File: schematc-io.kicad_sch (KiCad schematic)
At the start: 50 parts, among them IC1 AD8544ARUZ-REEL, J4 Conn_01x04, U3 SN65HVD232

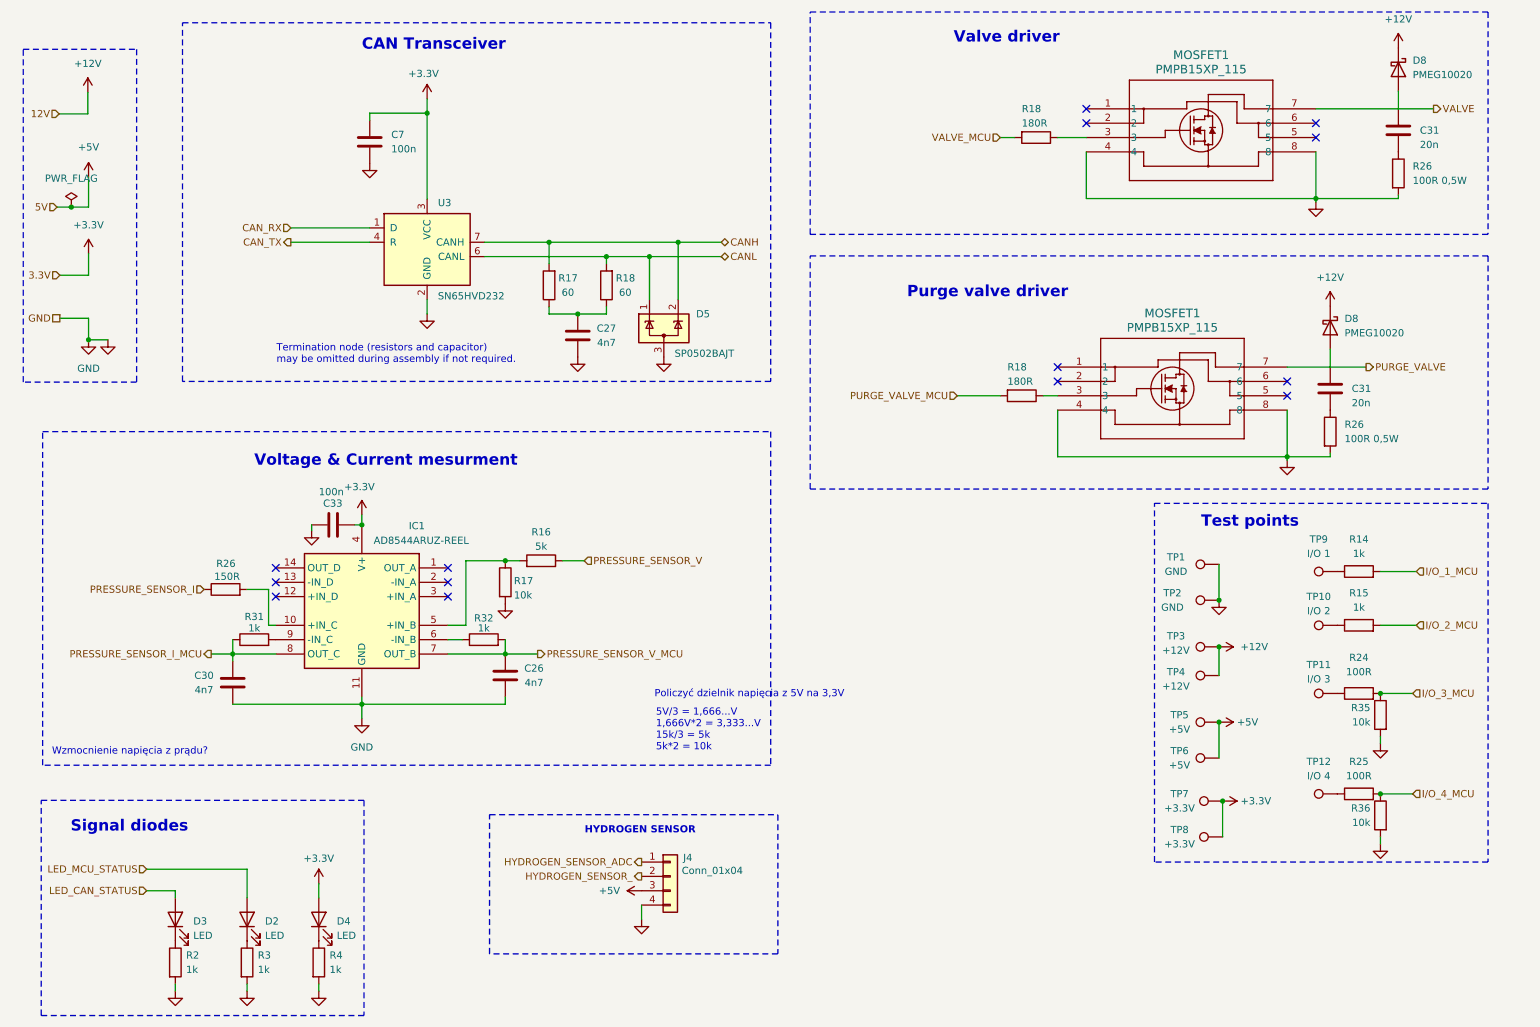
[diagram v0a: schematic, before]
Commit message: Adding motor driver unit
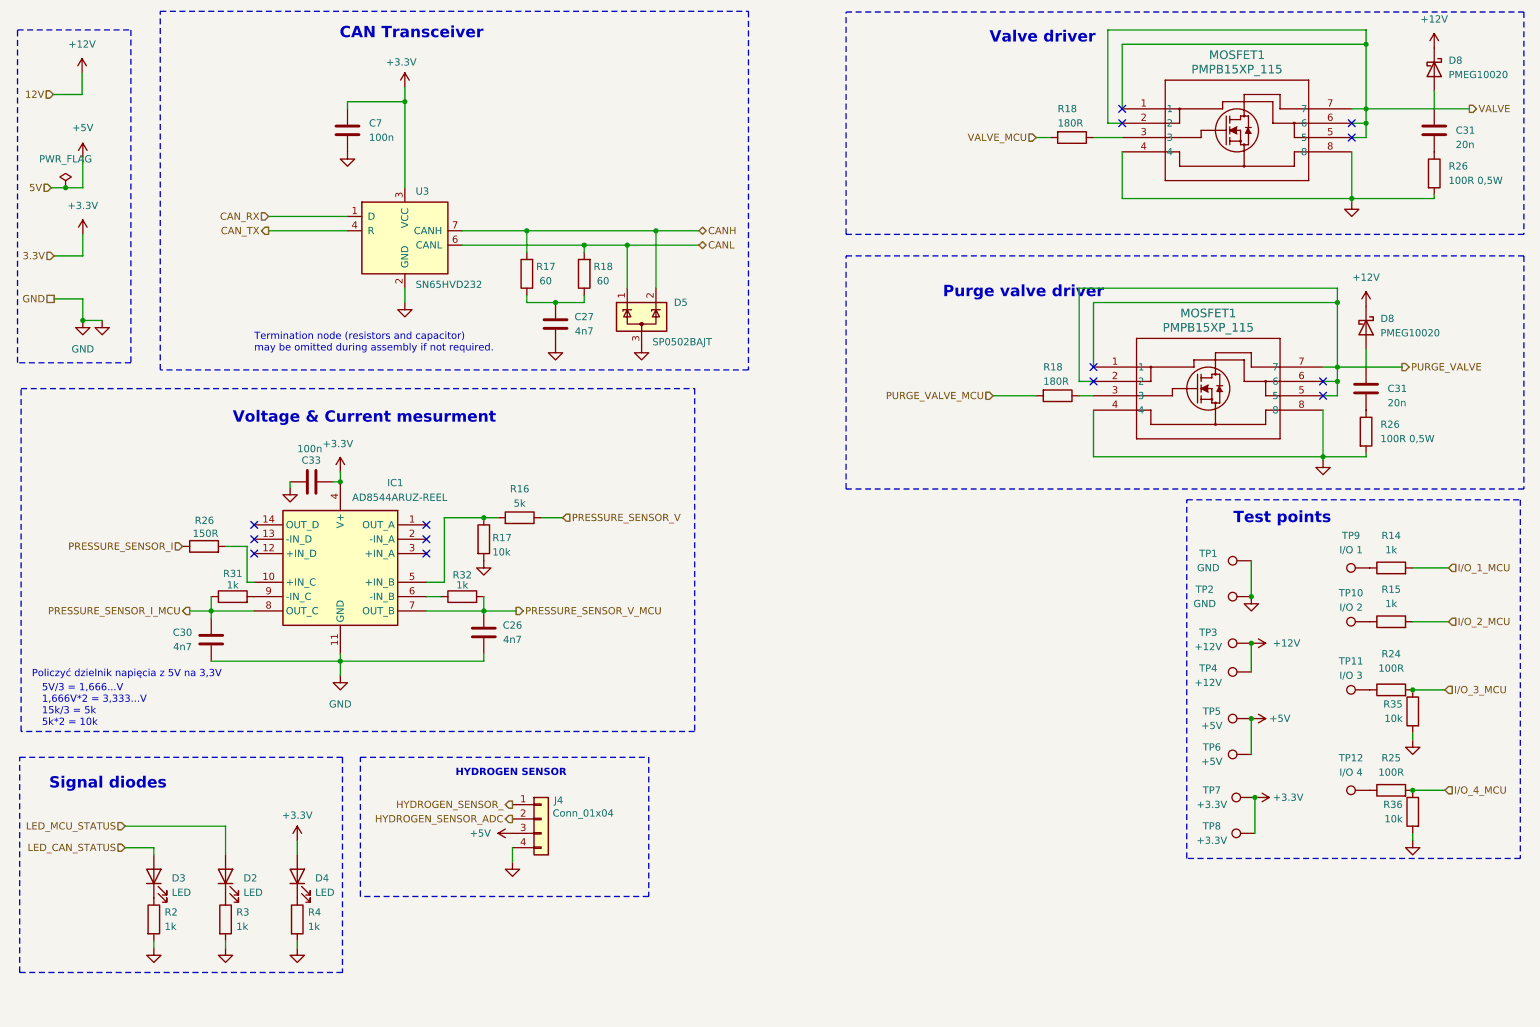
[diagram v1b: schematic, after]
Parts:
- D8: footprint Diode_SMD:DIOAD1414W86L464D238 -> Diode_SMD:PMEG10020ELR
- R18, R2, R26, R3, R4: footprint LED_SMD:LED_1206_3216Metric -> Resistor_SMD:R_1206_3216Metric
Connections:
- net HYDROGEN_SENSOR_: now also J4.1 (Pin_1); no longer J4.2 (Pin_2)
- net HYDROGEN_SENSOR_ADC: now also J4.2 (Pin_2); no longer J4.1 (Pin_1)
- net PURGE_VALVE: now also MOSFET1.1, MOSFET1.2, MOSFET1.5, MOSFET1.6
- net VALVE: now also MOSFET1.1, MOSFET1.2, MOSFET1.5, MOSFET1.6
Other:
- note removed: "Wzmocnienie napięcia z prądu?"
- moved on the sheet: C26, C27, C30, C31, C33, C7, D2, D3, D4, D5, D8, IC1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
